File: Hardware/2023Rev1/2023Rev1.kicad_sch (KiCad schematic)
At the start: 98 parts, among them J1 Conn_01x09, J2 Conn_01x09, J3 Conn_01x04, J4 Conn_01x03, Q1 Q_NMOS_GDS, Q2 Q_NMOS_DGS, SW1 SW_SPDT, U1 Teensy4.1_DEV-16771, U10 LT1910, U3 Opamp_Dual, U4 ACS758xCB-200B-PFF, U5 Opamp_Dual, U6 OKI, U7 Opamp_Dual, U8 Opamp_Dual, U9 TSR_1-2450

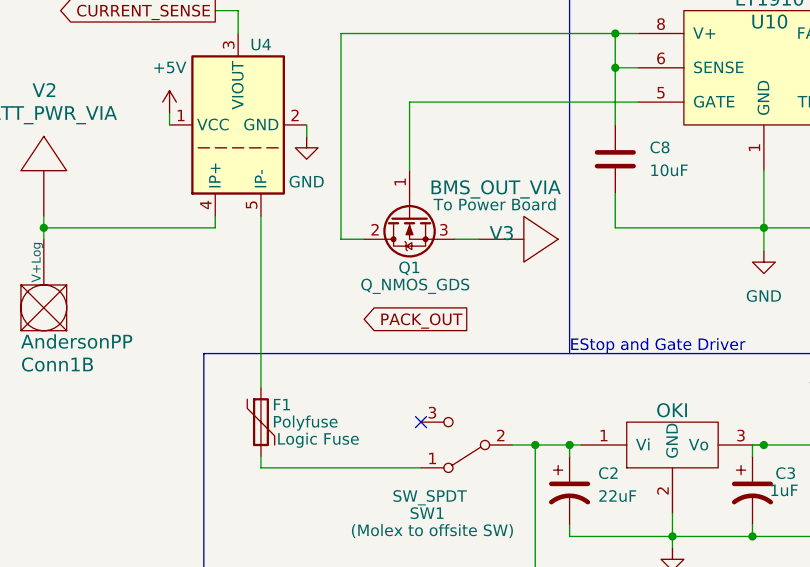
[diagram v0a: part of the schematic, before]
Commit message: more grid fixes
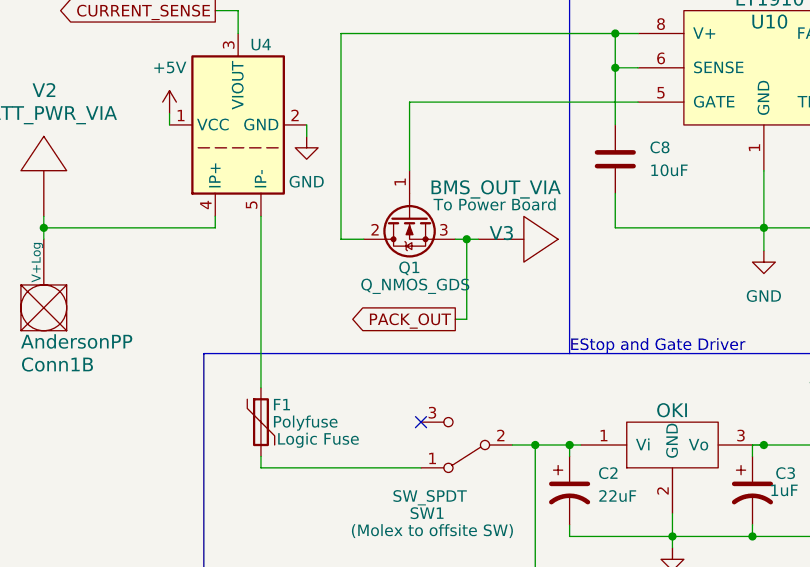
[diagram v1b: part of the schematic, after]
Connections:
- net PACK_OUT: now also Q1.3 (S), V3.1
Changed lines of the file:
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@@
   (junction (at 163.83 149.86) (diameter 0) (color 0 0 0 0)
+  )
+  (junction (at 243.84 40.64) (diameter 0) (color 0 0 0 0)
   )
   (junction (at 76.2 165.1) (diameter 0) (color 0 0 0 0)
@@
     (stroke (width 0) (type default) (color 0 0 0 0))
   )
+  (wire (pts (xy 243.84 40.64) (xy 243.84 49.53))
+    (stroke (width 0) (type default) (color 0 0 0 0))
+  )
   (wire (pts (xy 17.78 180.34) (xy 24.13 180.34))
     (stroke (width 0) (type default) (color 0 0 0 0))
@@
     (stroke (width 0) (type default) (color 0 0 0 0))
   )
-  (wire (pts (xy 242.57 40.64) (xy 245.11 40.64))
+  (wire (pts (xy 242.57 40.64) (xy 243.84 40.64))
     (stroke (width 0) (type default) (color 0 0 0 0))
   )
@@
     (stroke (width 0) (type default) (color 0 0 0 0))
   )
+  (wire (pts (xy 242.57 49.53) (xy 243.84 49.53))
+    (stroke (width 0) (type default) (color 0 0 0 0))
+  )
   (wire (pts (xy 325.12 62.23) (xy 334.01 62.23))
     (stroke (width 0) (type default) (color 0 0 0 0))
@@
   )
   (wire (pts (xy 210.82 26.67) (xy 210.82 27.94))
+    (stroke (width 0) (type default) (color 0 0 0 0))
+  )
+  (wire (pts (xy 243.84 40.64) (xy 245.11 40.64))
     (stroke (width 0) (type default) (color 0 0 0 0))
   )
@@
     )
   )
-  (global_label "PACK_OUT" (shape output) (at 243.84 49.53 180) (fields_autoplaced)
-    (effects (font (size 1.27 1.27)) (justify right))
-    (property "Intersheet References" "${INTERSHEET_REFS}" (id 0) (at 231.9321 49.6094 0)
-      (effects (font (size 1.27 1.27)) (justify right) hide)
-    )
+  (global_label "PACK_OUT" (shape output) (at 242.57 49.53 180) (fields_autoplaced)
+    (effects (font (size 1.27 1.27)) (justify right))
+    (property "Intersheet References" "${INTERSHEET_REFS}" (id 0) (at 230.6621 49.6094 0)
+      (effects (font (size 1.27 1.27)) (justify right) hide)
+    )
